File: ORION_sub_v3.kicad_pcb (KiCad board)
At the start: 2 copper layers, 45 x 75 mm, 70 parts, among them J1 Conn_01x02, J10 Conn_01x01, J11 Conn_01x05, J12 Conn_01x04, J2 Conn_01x03, J3 Conn_01x04, J4 Conn_01x02, J5 Conn_01x01, J6 Conn_01x04, J7 Conn_01x03, J8 Conn_01x04, J9 Conn_01x01, P1 CONN_01X06, Q1 2SC4213, SW1 SW_Push, SW2 SW_Push, SW3 SW_Push, SW4 SW_Push, SW5 SW_Push, U1 STM32F303CBTx, U2 MAX3051, U3 AZ1117-3.3, U4 BD9G101G, X1 ceralock

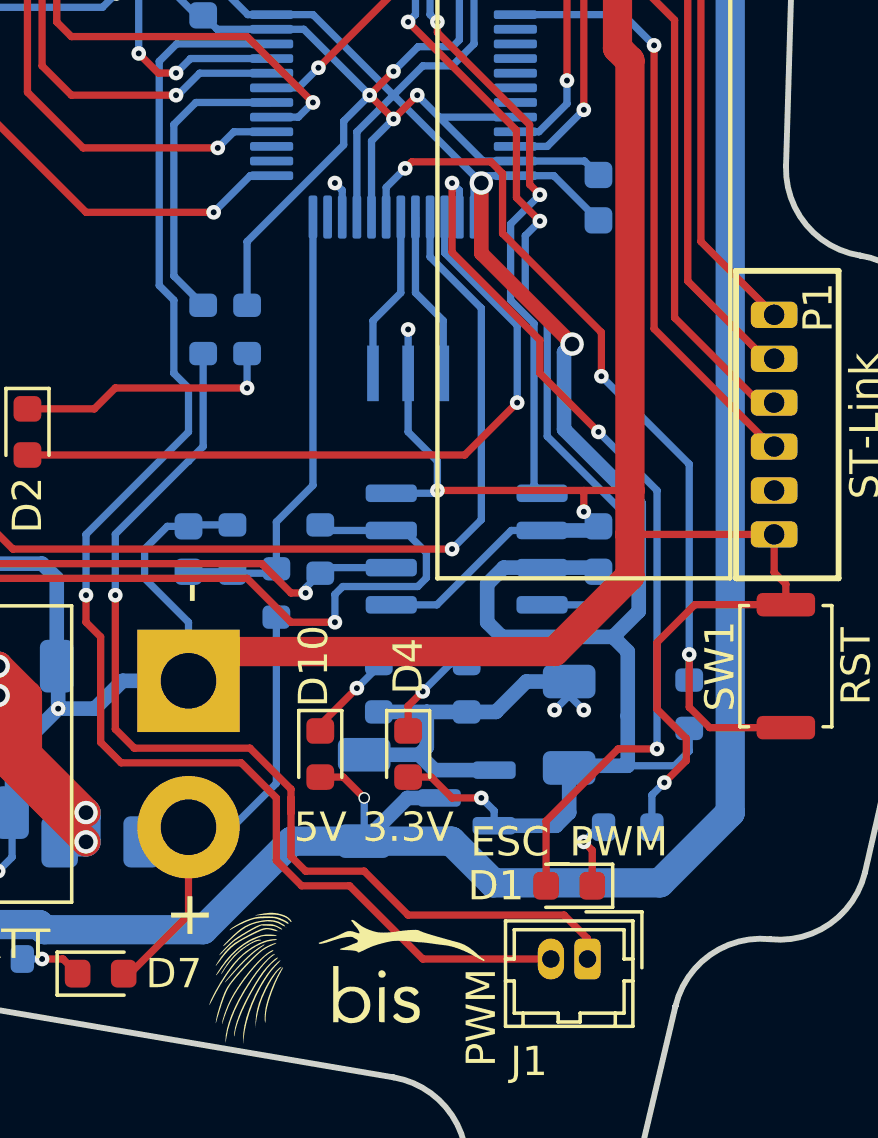
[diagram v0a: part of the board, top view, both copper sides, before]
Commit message: 更新
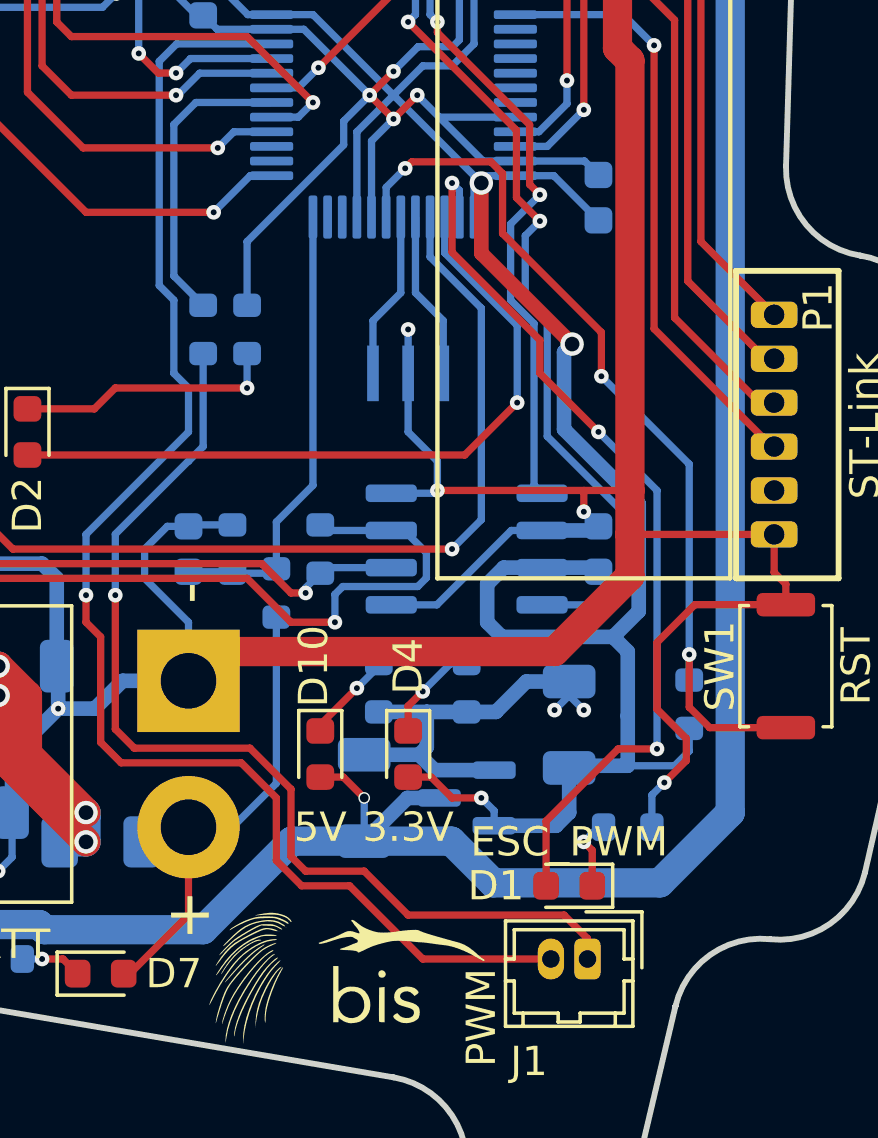
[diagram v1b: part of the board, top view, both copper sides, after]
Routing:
- net unconnected-(U1-PA0-Pad10): track 1.27 -> 0.00 mm, vias 1 -> 0
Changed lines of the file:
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@@
 	)
 	(segment
-		(start 126.625 107.5)
-		(end 126.625 106.8)
+		(start 116.5 101.7)
+		(end 116.5 104)
+		(width 0.25)
+		(layer "F.Cu")
+		(net 39)
+	)
+	(segment
+		(start 115.1 100.3)
+		(end 116.5 101.7)
+		(width 0.25)
+		(layer "F.Cu")
+		(net 39)
+	)
+	(segment
+		(start 110.5 99.65)
+		(end 111.15 100.3)
+		(width 0.25)
+		(layer "F.Cu")
+		(net 39)
+	)
+	(segment
+		(start 116.5 104)
+		(end 117 104.5)
+		(width 0.25)
+		(layer "F.Cu")
+		(net 39)
+	)
+	(segment
+		(start 119 104.5)
+		(end 120.5 106)
+		(width 0.25)
+		(layer "F.Cu")
+		(net 39)
+	)
+	(segment
+		(start 126.625 106.8)
+		(end 126.625 107.5)
+		(width 0.25)
+		(layer "F.Cu")
+		(net 39)
+	)
+	(segment
+		(start 117 104.5)
+		(end 119 104.5)
 		(width 0.25)
 		(layer "F.Cu")
@@
 	)
 	(segment
+		(start 120.5 106)
+		(end 125.825 106)
+		(width 0.25)
+		(layer "F.Cu")
+		(net 39)
+	)
+	(segment
 		(start 111.15 100.3)
 		(end 115.1 100.3)
@@
 	)
 	(segment
-		(start 126.625 106.8)
-		(end 125.825 106)
-		(width 0.25)
-		(layer "F.Cu")
-		(net 39)
-	)
-	(segment
-		(start 116.5 101.7)
-		(end 116.5 102.5)
-		(width 0.25)
-		(layer "F.Cu")
-		(net 39)
-	)
-	(segment
-		(start 116.5 104)
-		(end 117 104.5)
-		(width 0.25)
-		(layer "F.Cu")
-		(net 39)
-	)
-	(segment
-		(start 116.5 102.5)
-		(end 116.5 102.363604)
-		(width 0.25)
-		(layer "F.Cu")
-		(net 39)
-	)
-	(segment
-		(start 110.5 99.65)
-		(end 111.15 100.3)
-		(width 0.25)
-		(layer "F.Cu")
-		(net 39)
-	)
-	(segment
-		(start 116.5 102.363604)
-		(end 116.5 102)
-		(width 0.25)
-		(layer "F.Cu")
-		(net 39)
-	)
-	(segment
-		(start 116.5 102.5)
-		(end 116.5 104)
-		(width 0.25)
-		(layer "F.Cu")
-		(net 39)
-	)
-	(segment
-		(start 115.1 100.3)
-		(end 116.5 101.7)
-		(width 0.25)
-		(layer "F.Cu")
-		(net 39)
-	)
-	(segment
 		(start 125.825 106)
-		(end 120.5 106)
-		(width 0.25)
-		(layer "F.Cu")
-		(net 39)
-	)
-	(segment
-		(start 117 104.5)
-		(end 119 104.5)
-		(width 0.25)
-		(layer "F.Cu")
-		(net 39)
-	)
-	(segment
-		(start 120.5 106)
-		(end 119 104.5)
+		(end 126.625 106.8)
 		(width 0.25)
 		(layer "F.Cu")
@@
 		(net 57)
 	)
-	(via
-		(at 118 81)
-		(size 0.5)
-		(drill 0.2)
-		(layers "F.Cu" "B.Cu")
-		(net 66)
-	)
-	(segment
-		(start 118.25 81.25)
-		(end 118.25 82.1625)
-		(width 0.25)
-		(layer "B.Cu")
-		(net 66)
-	)
-	(segment
-		(start 118 81)
-		(end 118.25 81.25)
-		(width 0.25)
-		(layer "B.Cu")
-		(net 66)
-	)
-	(segment
+	(segment
